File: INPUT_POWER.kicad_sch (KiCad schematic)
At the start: 20 parts, among them Q1 PJA3401A_R1_00001, Q3 Q_Dual_NMOS_PMOS_G1S2G2D2S1D1, SW1 A6TN-1104, U5 TLV75533PDBV

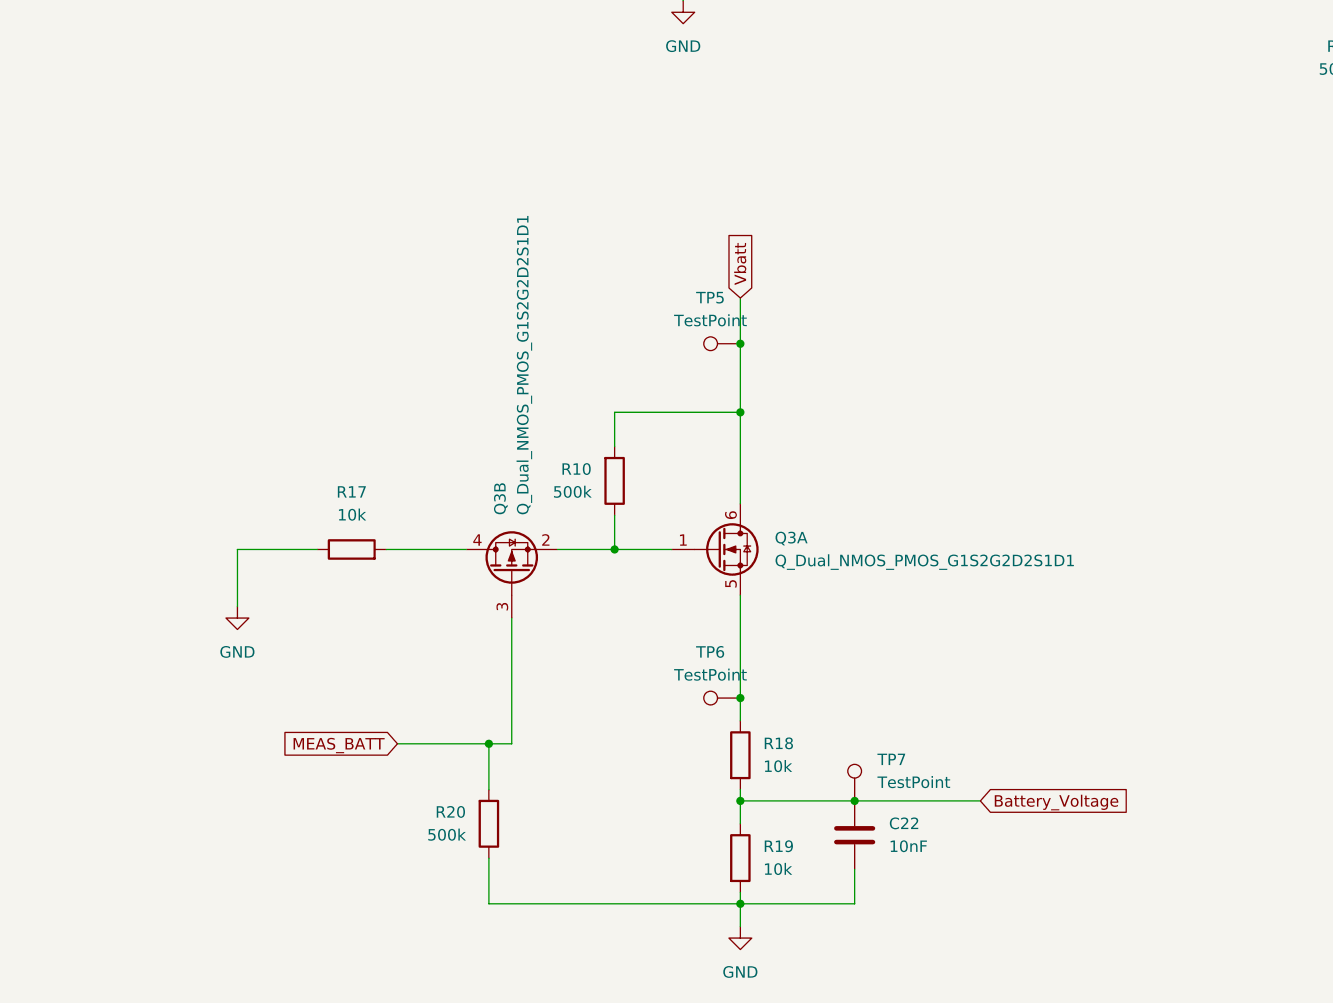
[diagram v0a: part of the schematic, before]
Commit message: finished board layout for AD revision
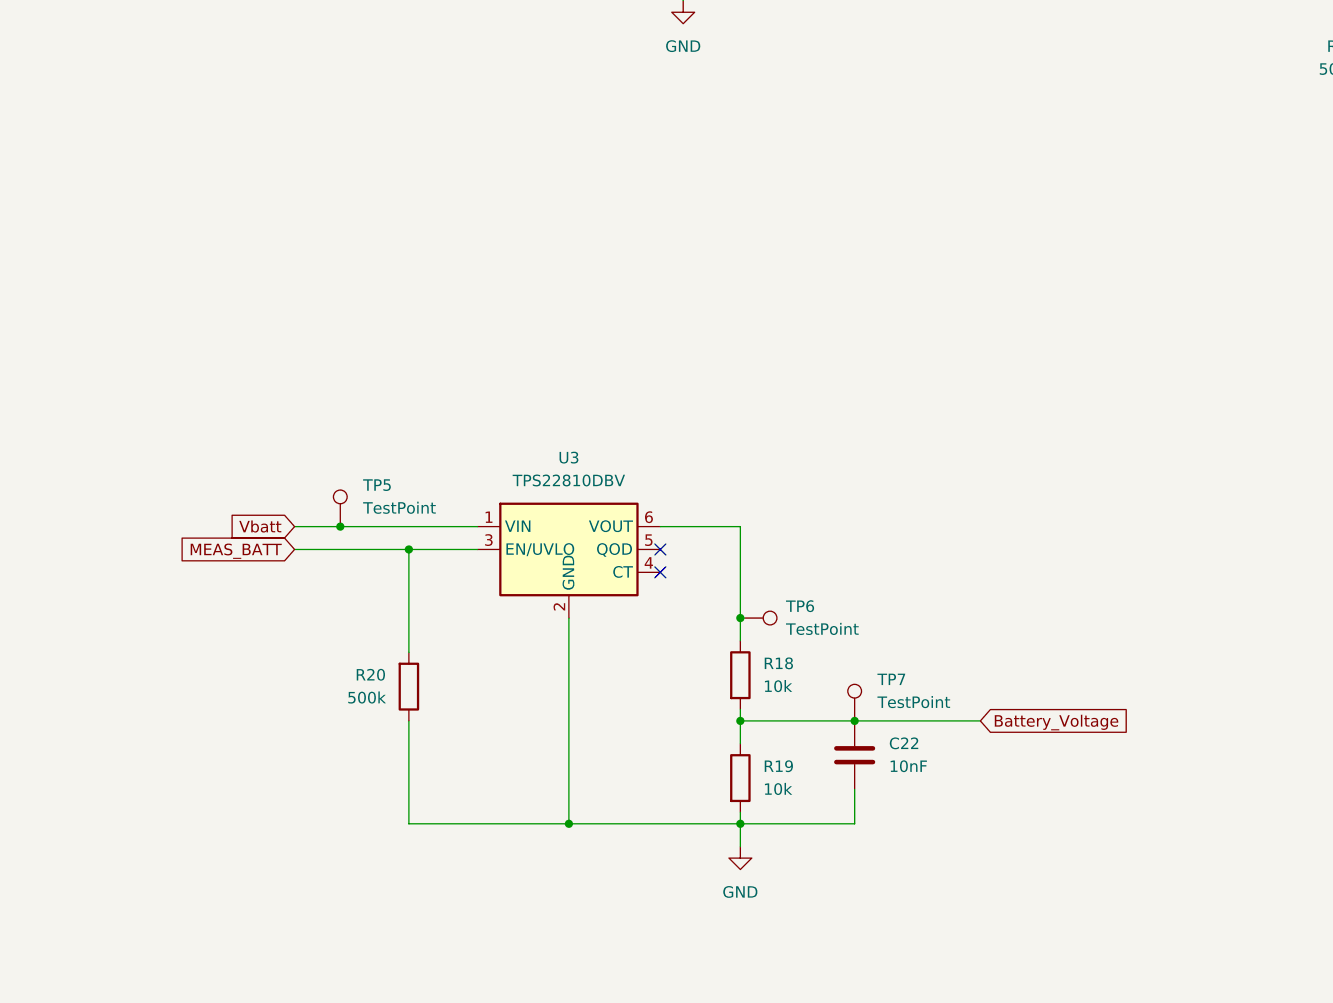
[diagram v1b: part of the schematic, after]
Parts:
- removed Q3: Q_Dual_NMOS_PMOS_G1S2G2D2S1D1, Package_SO:TSOP-6_1.65x3.05mm_P0.95mm, symbol Transistor_FET:Q_Dual_NMOS_PMOS_G1S2G2D2S1D1
- removed R10: 500k, Resistor_SMD:R_0805_2012Metric_Pad1.20x1.40mm_HandSolder, symbol Device:R
- removed R17: 10k, Resistor_SMD:R_0805_2012Metric_Pad1.20x1.40mm_HandSolder, symbol Device:R
- added U3: TPS22810DBV, Package_TO_SOT_SMD:SOT-23-6, symbol Power_Management:TPS22810DBV
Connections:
- net GND: now also U3.2 (GND)
- net MEAS_BATT: now also U3.3 (EN/UVLO)
- net Vbatt: now also U3.1 (VIN)
- net at R18.1, TP6.1: now also U3.6 (VOUT)
- no-connect marks 0 -> 2
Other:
- moved on the sheet: C22, R18, R19, R20, TP5, TP6, TP7
